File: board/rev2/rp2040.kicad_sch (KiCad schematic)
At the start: 37 parts, among them U8 TLV74311, U9 RP2354B, Y1 ABM8-272-T3

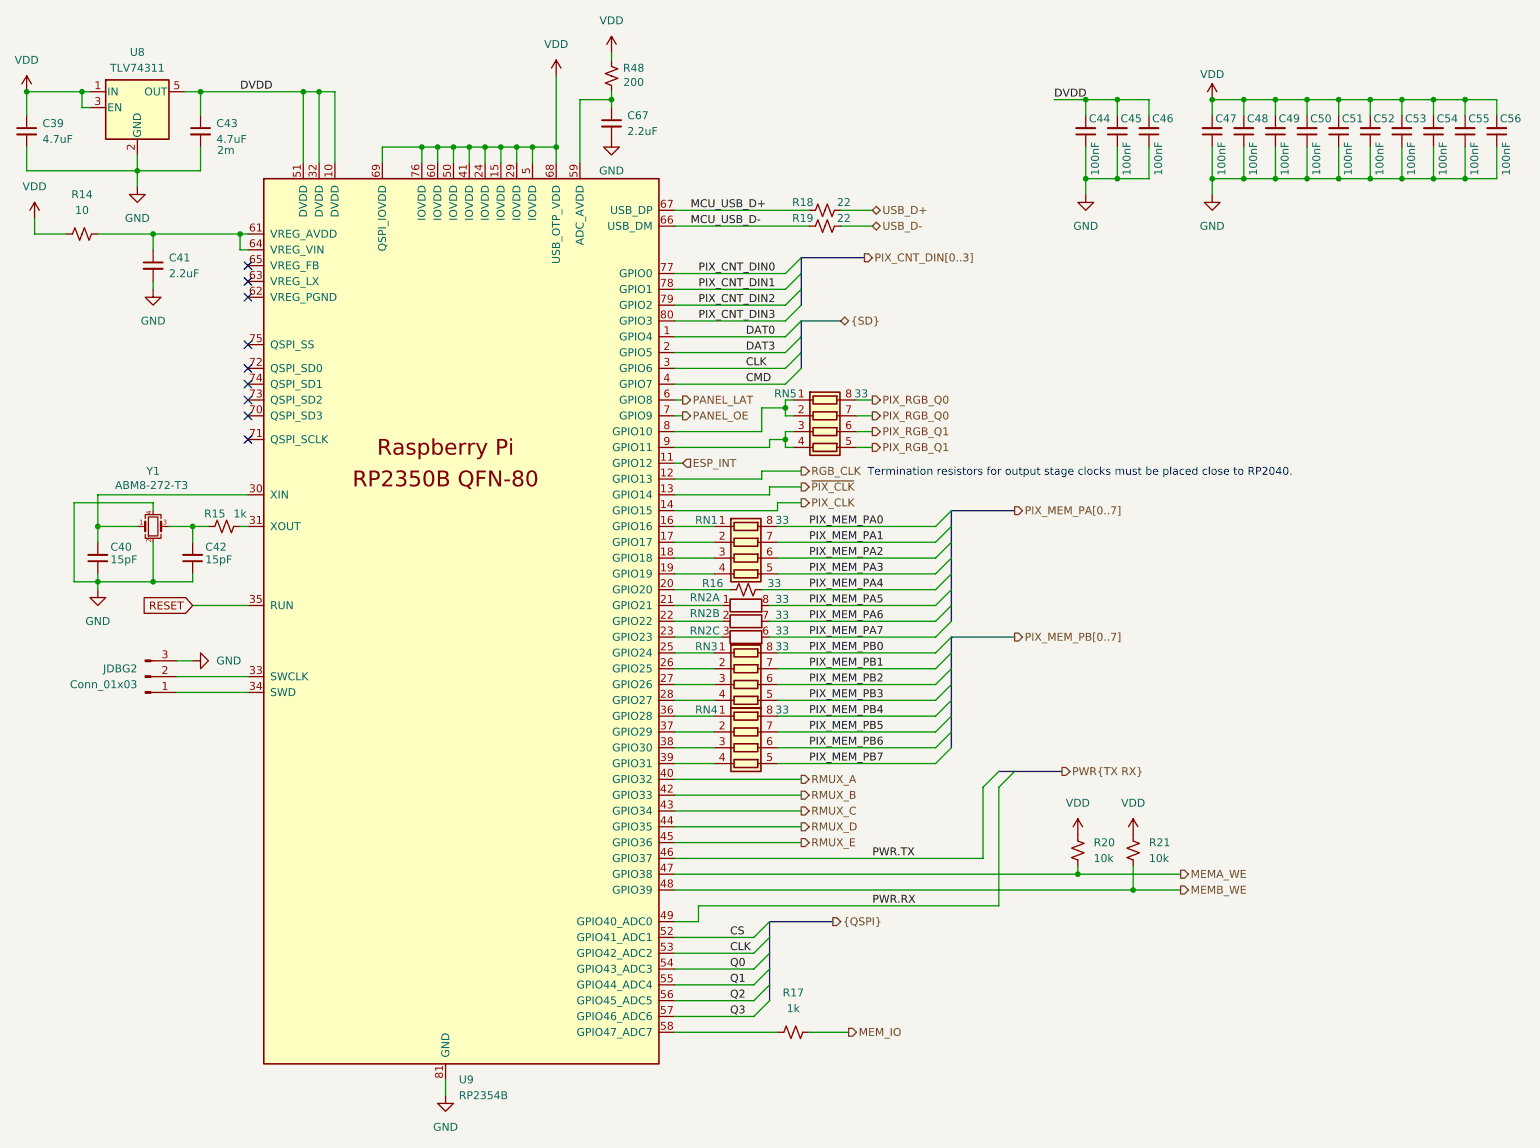
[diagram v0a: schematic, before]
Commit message: 3.3V LDO
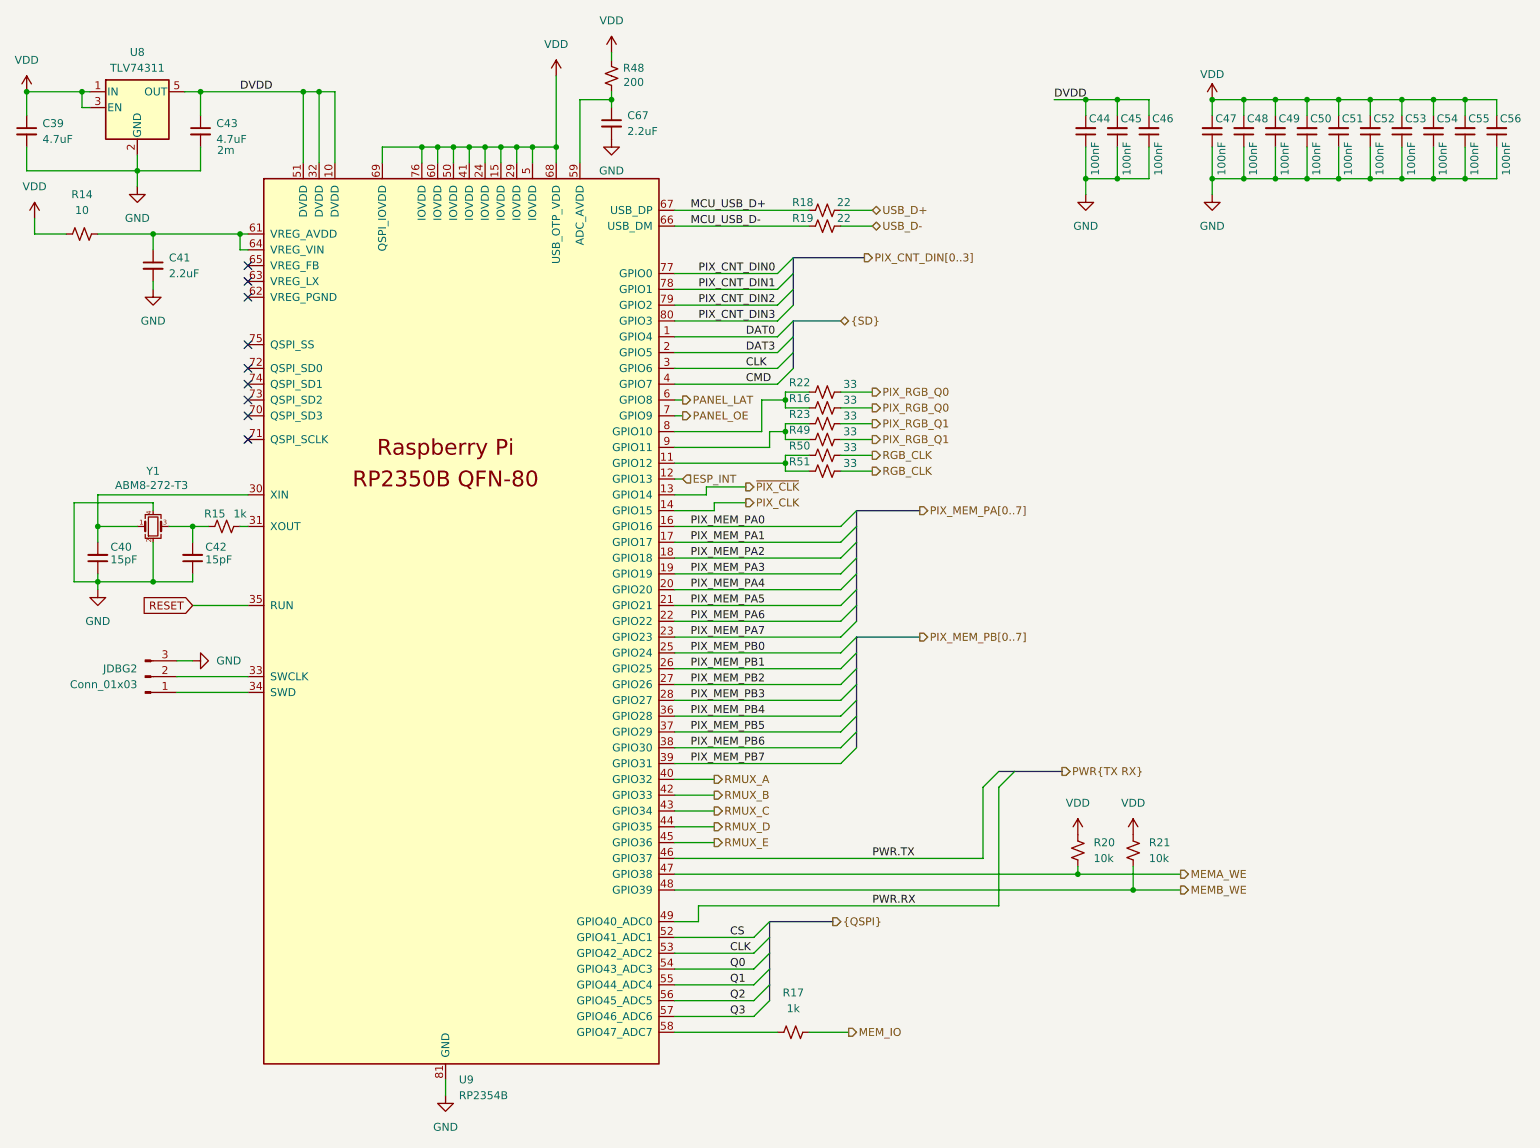
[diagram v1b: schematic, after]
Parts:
- removed RN1, RN3, RN4, RN5: 33, RN_SMD:R_Array_Flat_4x0201, symbol Device:R_Pack04
- removed RN2: 33, RN_SMD:R_Array_Flat_4x0201, symbol Device:R_Pack04_Split
- added R22, R23, R49, R50, R51: 33, Resistor_SMD:R_0402_1005Metric, symbol Device:R_Small_US
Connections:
- net ESP_INT: now also U9.12 (GPIO13); no longer U9.11 (GPIO12)
- net PIX_MEM_PA0: now also U9.16 (GPIO16)
- net PIX_MEM_PA1: now also U9.17 (GPIO17)
- net PIX_MEM_PA2: now also U9.18 (GPIO18)
- net PIX_MEM_PA3: now also U9.19 (GPIO19)
- net PIX_MEM_PA4: now also U9.20 (GPIO20); no longer R16.2
- net PIX_MEM_PA5: now also U9.21 (GPIO21)
- net PIX_MEM_PA6: now also U9.22 (GPIO22)
- net PIX_MEM_PA7: now also U9.23 (GPIO23)
- net PIX_MEM_PB0: now also U9.25 (GPIO24)
- net PIX_MEM_PB1: now also U9.26 (GPIO25)
- net PIX_MEM_PB2: now also U9.27 (GPIO26)
- net PIX_MEM_PB3: now also U9.28 (GPIO27)
- net PIX_MEM_PB4: now also U9.36 (GPIO28)
- net PIX_MEM_PB5: now also U9.37 (GPIO29)
- net PIX_MEM_PB6: now also U9.38 (GPIO30)
- net PIX_MEM_PB7: now also U9.39 (GPIO31)
- net PIX_RGB_Q0: now also R16.2, R22.2
- net PIX_RGB_Q1: now also R23.2, R49.2
- net RGB_CLK: now also R50.2, R51.2; no longer U9.12 (GPIO13)
- net at R16.1: now also U9.8 (GPIO10), R22.1; no longer U9.20 (GPIO20)
- net at U9.9 (GPIO11): now also R23.1, R49.1
- new net: R50.1, R51.1, U9.11 (GPIO12)
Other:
- note removed: "Termination resistors for output stage clocks must be placed close to RP2040."
